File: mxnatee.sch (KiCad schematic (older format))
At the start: 45 parts, among them U1 ProMicro, U2 TRRS

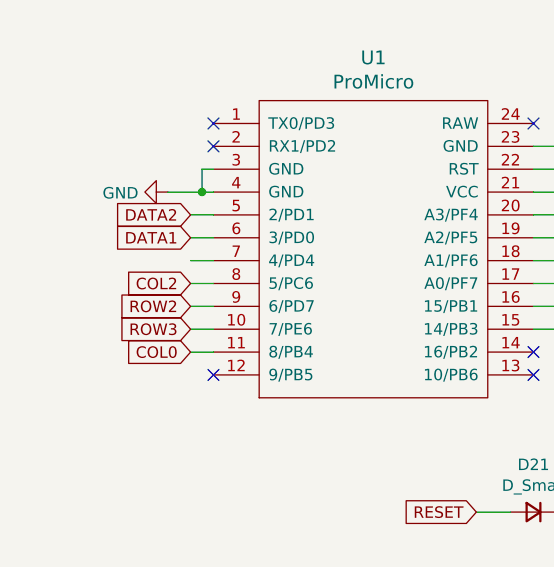
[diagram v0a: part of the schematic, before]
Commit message: Initial attempt at doing cool edge cuts
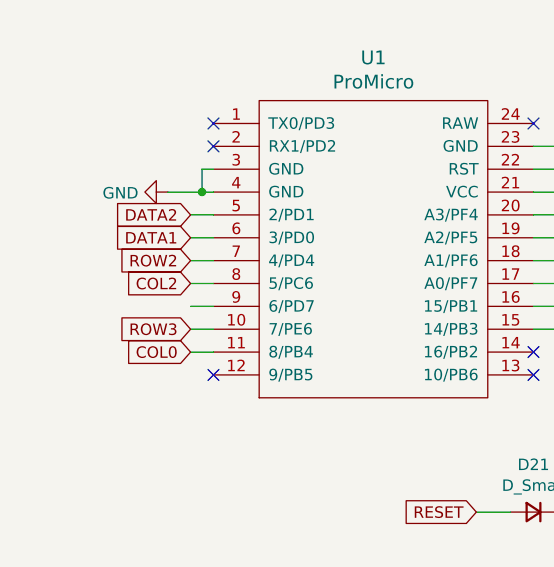
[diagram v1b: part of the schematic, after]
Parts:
- D1, D10, D11, D12, D13, D14, D15, D16, D17, D18, D19, D2, D21, D3, D4, D5, D6, D7, D8, D9: footprint random-keyboard-parts:D_SOD-123-Pretty -> Keebio-Parts:D_SOD123
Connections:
- net ROW2: now also U1.7 (4/PD4); no longer U1.9 (6/PD7)
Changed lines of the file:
@@
 F 0 "D21" H 3450 3693 50  0000 C CNN
 F 1 "D_Small" H 3450 3784 50  0000 C CNN
-F 2 "random-keyboard-parts:D_SOD-123-Pretty" V 3450 3900 50  0001 C CNN
+F 2 "Keebio-Parts:D_SOD123" V 3450 3900 50  0001 C CNN
 F 3 "~" V 3450 3900 50  0001 C CNN
 	1    3450 3900
@@
 Text GLabel 3600 2700 2    50   Input ~ 0
 ROW1
-Text GLabel 1950 3000 0    50   Input ~ 0
+Text GLabel 1950 2800 0    50   Input ~ 0
 ROW2
 Wire Wire Line
@@
 F 0 "D1" V 6204 2270 50  0000 L CNN
 F 1 "D_Small" V 6295 2270 50  0000 L CNN
-F 2 "random-keyboard-parts:D_SOD-123-Pretty" V 6250 2200 50  0001 C CNN
+F 2 "Keebio-Parts:D_SOD123" V 6250 2200 50  0001 C CNN
 F 3 "~" V 6250 2200 50  0001 C CNN
 	1    6250 2200
@@
 F 0 "D2" V 6654 2270 50  0000 L CNN
 F 1 "D_Small" V 6745 2270 50  0000 L CNN
-F 2 "random-keyboard-parts:D_SOD-123-Pretty" V 6700 2200 50  0001 C CNN
+F 2 "Keebio-Parts:D_SOD123" V 6700 2200 50  0001 C CNN
 F 3 "~" V 6700 2200 50  0001 C CNN
 	1    6700 2200
@@
 F 0 "D3" V 5754 2820 50  0000 L CNN
 F 1 "D_Small" V 5845 2820 50  0000 L CNN
-F 2 "random-keyboard-parts:D_SOD-123-Pretty" V 5800 2750 50  0001 C CNN
+F 2 "Keebio-Parts:D_SOD123" V 5800 2750 50  0001 C CNN
 F 3 "~" V 5800 2750 50  0001 C CNN
 	1    5800 2750
@@
 F 0 "D4" V 6204 2820 50  0000 L CNN
 F 1 "D_Small" V 6295 2820 50  0000 L CNN
-F 2 "random-keyboard-parts:D_SOD-123-Pretty" V 6250 2750 50  0001 C CNN
+F 2 "Keebio-Parts:D_SOD123" V 6250 2750 50  0001 C CNN
 F 3 "~" V 6250 2750 50  0001 C CNN
 	1    6250 2750
@@
 F 0 "D5" V 6654 2820 50  0000 L CNN
 F 1 "D_Small" V 6745 2820 50  0000 L CNN
-F 2 "random-keyboard-parts:D_SOD-123-Pretty" V 6700 2750 50  0001 C CNN
+F 2 "Keebio-Parts:D_SOD123" V 6700 2750 50  0001 C CNN
 F 3 "~" V 6700 2750 50  0001 C CNN
 	1    6700 2750
@@
 F 0 "D6" V 7154 2820 50  0000 L CNN
 F 1 "D_Small" V 7245 2820 50  0000 L CNN
-F 2 "random-keyboard-parts:D_SOD-123-Pretty" V 7200 2750 50  0001 C CNN
+F 2 "Keebio-Parts:D_SOD123" V 7200 2750 50  0001 C CNN
 F 3 "~" V 7200 2750 50  0001 C CNN
 	1    7200 2750
@@
 F 0 "D7" V 5754 3370 50  0000 L CNN
 F 1 "D_Small" V 5845 3370 50  0000 L CNN
-F 2 "random-keyboard-parts:D_SOD-123-Pretty" V 5800 3300 50  0001 C CNN
+F 2 "Keebio-Parts:D_SOD123" V 5800 3300 50  0001 C CNN
 F 3 "~" V 5800 3300 50  0001 C CNN
 	1    5800 3300
@@
 F 0 "D8" V 6204 3370 50  0000 L CNN
 F 1 "D_Small" V 6295 3370 50  0000 L CNN
-F 2 "random-keyboard-parts:D_SOD-123-Pretty" V 6250 3300 50  0001 C CNN
+F 2 "Keebio-Parts:D_SOD123" V 6250 3300 50  0001 C CNN
 F 3 "~" V 6250 3300 50  0001 C CNN
 	1    6250 3300
@@
 F 0 "D9" V 6654 3370 50  0000 L CNN
 F 1 "D_Small" V 6745 3370 50  0000 L CNN
-F 2 "random-keyboard-parts:D_SOD-123-Pretty" V 6700 3300 50  0001 C CNN
+F 2 "Keebio-Parts:D_SOD123" V 6700 3300 50  0001 C CNN
 F 3 "~" V 6700 3300 50  0001 C CNN
 	1    6700 3300
@@
 F 0 "D10" V 7154 3370 50  0000 L CNN
 F 1 "D_Small" V 7245 3370 50  0000 L CNN
-F 2 "random-keyboard-parts:D_SOD-123-Pretty" V 7200 3300 50  0001 C CNN
+F 2 "Keebio-Parts:D_SOD123" V 7200 3300 50  0001 C CNN
 F 3 "~" V 7200 3300 50  0001 C CNN
 	1    7200 3300
@@
 F 0 "D11" V 5354 3920 50  0000 L CNN
 F 1 "D_Small" V 5445 3920 50  0000 L CNN
-F 2 "random-keyboard-parts:D_SOD-123-Pretty" V 5400 3850 50  0001 C CNN
+F 2 "Keebio-Parts:D_SOD123" V 5400 3850 50  0001 C CNN
 F 3 "~" V 5400 3850 50  0001 C CNN
 	1    5400 3850
@@
 F 0 "D12" V 6204 3920 50  0000 L CNN
 F 1 "D_Small" V 6295 3920 50  0000 L CNN
-F 2 "random-keyboard-parts:D_SOD-123-Pretty" V 6250 3850 50  0001 C CNN
+F 2 "Keebio-Parts:D_SOD123" V 6250 3850 50  0001 C CNN
 F 3 "~" V 6250 3850 50  0001 C CNN
 	1    6250 3850
@@
 F 0 "D13" V 6654 3920 50  0000 L CNN
 F 1 "D_Small" V 6745 3920 50  0000 L CNN
-F 2 "random-keyboard-parts:D_SOD-123-Pretty" V 6700 3850 50  0001 C CNN
+F 2 "Keebio-Parts:D_SOD123" V 6700 3850 50  0001 C CNN
 F 3 "~" V 6700 3850 50  0001 C CNN
 	1    6700 3850
@@
 F 0 "D14" V 7154 3920 50  0000 L CNN
 F 1 "D_Small" V 7245 3920 50  0000 L CNN
-F 2 "random-keyboard-parts:D_SOD-123-Pretty" V 7200 3850 50  0001 C CNN
+F 2 "Keebio-Parts:D_SOD123" V 7200 3850 50  0001 C CNN
 F 3 "~" V 7200 3850 50  0001 C CNN
 	1    7200 3850
@@
 F 0 "D15" V 5354 4420 50  0000 L CNN
 F 1 "D_Small" V 5445 4420 50  0000 L CNN
-F 2 "random-keyboard-parts:D_SOD-123-Pretty" V 5400 4350 50  0001 C CNN
+F 2 "Keebio-Parts:D_SOD123" V 5400 4350 50  0001 C CNN
 F 3 "~" V 5400 4350 50  0001 C CNN
 	1    5400 4350
@@
 F 0 "D16" V 5754 4420 50  0000 L CNN
 F 1 "D_Small" V 5845 4420 50  0000 L CNN
-F 2 "random-keyboard-parts:D_SOD-123-Pretty" V 5800 4350 50  0001 C CNN
+F 2 "Keebio-Parts:D_SOD123" V 5800 4350 50  0001 C CNN
 F 3 "~" V 5800 4350 50  0001 C CNN
 	1    5800 4350
@@
 F 0 "D17" V 6204 4420 50  0000 L CNN
 F 1 "D_Small" V 6295 4420 50  0000 L CNN
-F 2 "random-keyboard-parts:D_SOD-123-Pretty" V 6250 4350 50  0001 C CNN
+F 2 "Keebio-Parts:D_SOD123" V 6250 4350 50  0001 C CNN
 F 3 "~" V 6250 4350 50  0001 C CNN
 	1    6250 4350
@@
 F 0 "D18" V 6654 4420 50  0000 L CNN
 F 1 "D_Small" V 6745 4420 50  0000 L CNN
-F 2 "random-keyboard-parts:D_SOD-123-Pretty" V 6700 4350 50  0001 C CNN
+F 2 "Keebio-Parts:D_SOD123" V 6700 4350 50  0001 C CNN
 F 3 "~" V 6700 4350 50  0001 C CNN
 	1    6700 4350
@@
 F 0 "D19" V 7154 4420 50  0000 L CNN
 F 1 "D_Small" V 7245 4420 50  0000 L CNN
-F 2 "random-keyboard-parts:D_SOD-123-Pretty" V 7200 4350 50  0001 C CNN
+F 2 "Keebio-Parts:D_SOD123" V 7200 4350 50  0001 C CNN
 F 3 "~" V 7200 4350 50  0001 C CNN
 	1    7200 4350
